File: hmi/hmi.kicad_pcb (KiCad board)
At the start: 2 copper layers, 38 x 50 mm, 23 parts, among them J1 sensor, J2 parachute, J3 aerofrein

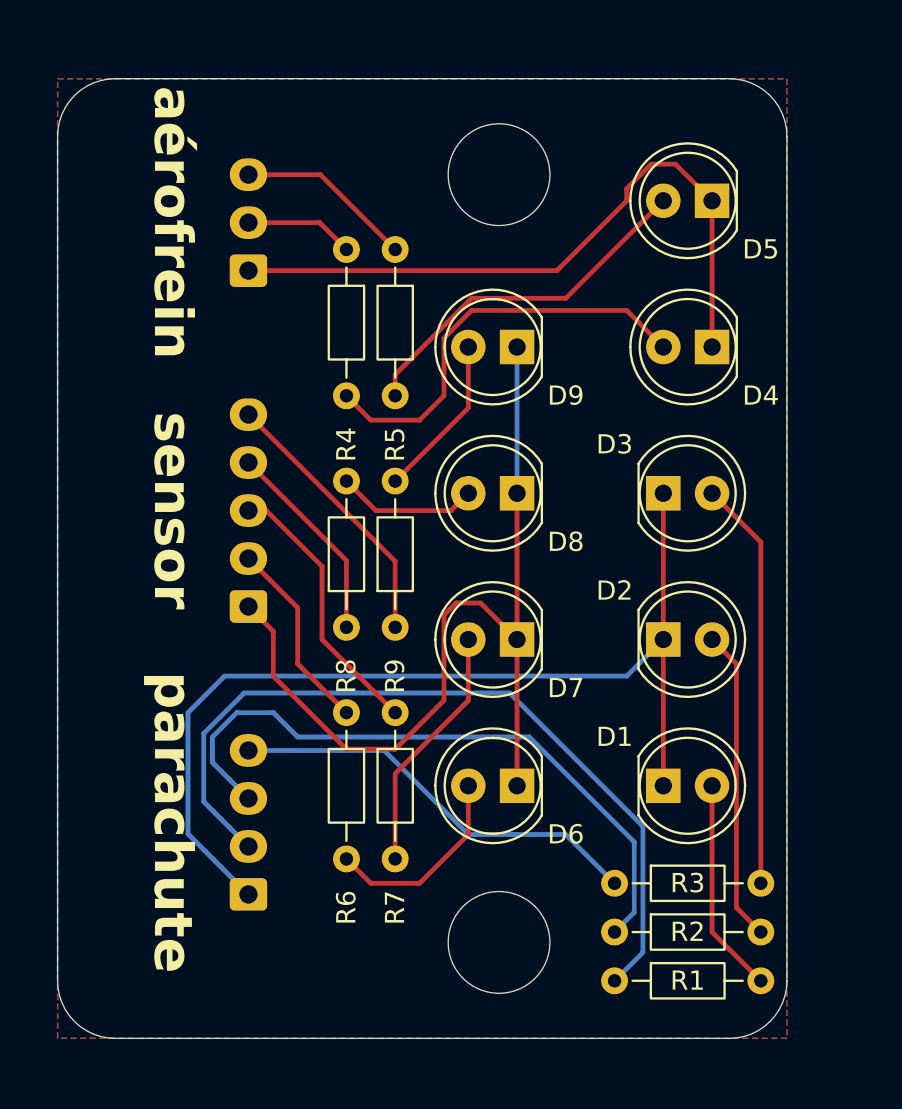
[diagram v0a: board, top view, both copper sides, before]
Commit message: hmi full revision
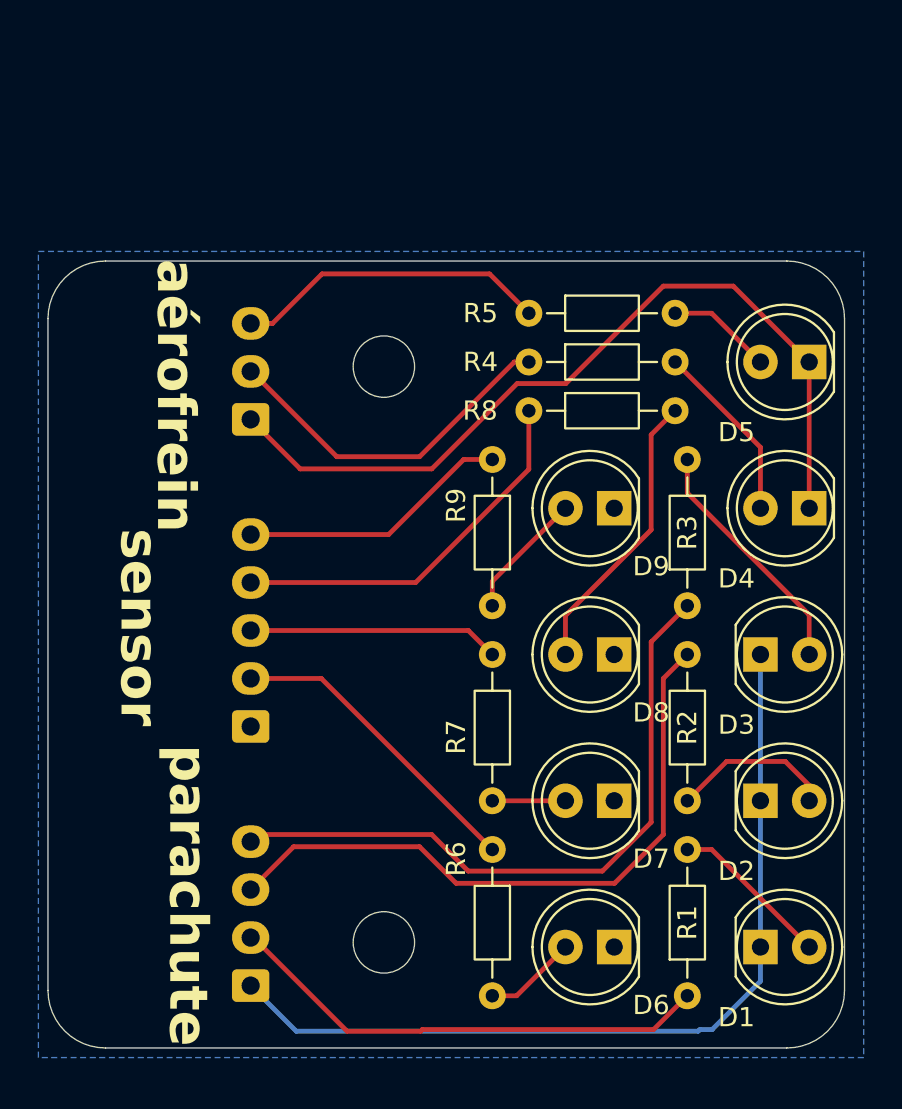
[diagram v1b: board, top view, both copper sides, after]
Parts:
- H1, H2: value MountingHole_5.3mm_M5_ISO14580 -> MountingHole_3.2mm_M3; footprint MountingHole:MountingHole_5.3mm_M5_ISO14580 -> MountingHole:MountingHole_3.2mm_M3
- moved R3 14.9 mm to (163.8, 107.5), turned to 90 degrees
- moved R2 14.9 mm to (163.8, 110.0), turned to -90 degrees
- moved R8 14.8 mm to (155.6, 97.3), turned to 0 degrees
- moved H1 11.7 mm to (148.0, 95.0)
- moved R4 11.2 mm to (155.6, 94.8), turned to 0 degrees
- moved R6 10.4 mm to (153.7, 120.2)
- moved R9 10.1 mm to (153.7, 99.8), turned to -90 degrees
- moved D2 9.81 mm to (167.6, 117.6)
- moved D3 9.81 mm to (167.6, 110.0)
- moved D5 9.81 mm to (170.2, 94.8)
- moved D7 9.81 mm to (160.0, 117.6)
- moved D8 9.81 mm to (160.0, 110.0)
- moved D1 9.81 mm to (167.6, 125.2)
- moved D4 9.81 mm to (170.2, 102.4)
- moved D6 9.81 mm to (160.0, 125.2)
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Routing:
- net GND3: track 47.8 -> 0.00 mm
- net Net-(J2-Pin_2): track 42.1 -> 25.5 mm
- net Net-(D5-A): track 18.8 -> 5.50 mm
- net Net-(J2-Pin_4): track 21.9 -> 34.9 mm
- net Net-(J3-Pin_2): track 5.68 -> 18.4 mm
- net Net-(D4-A): track 22.0 -> 9.46 mm
- net Net-(J1-Pin_4): track 10.7 -> 20.0 mm
- net Net-(D7-A): track 13.0 -> 3.81 mm
- net Net-(D3-A): track 21.4 -> 12.8 mm
- net GND1: track 35.2 -> 43.4 mm
- net Net-(D2-A): track 16.3 -> 8.52 mm
- net Net-(D8-A): track 7.36 -> 15.1 mm
- net Net-(J3-Pin_3): track 9.26 -> 16.4 mm
- net GND2: track 52.4 -> 45.6 mm
- net Net-(J1-Pin_2): track 10.1 -> 16.3 mm
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- added copper zone on B.Cu, net GND3
- removed copper zone on B.Cu, net (none)
- removed copper zone on F.Cu, net (none)
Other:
- board size 38 x 50 mm -> 41.5 x 41 mm
